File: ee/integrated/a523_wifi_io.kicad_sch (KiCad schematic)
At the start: 7 parts, among them U201 A523

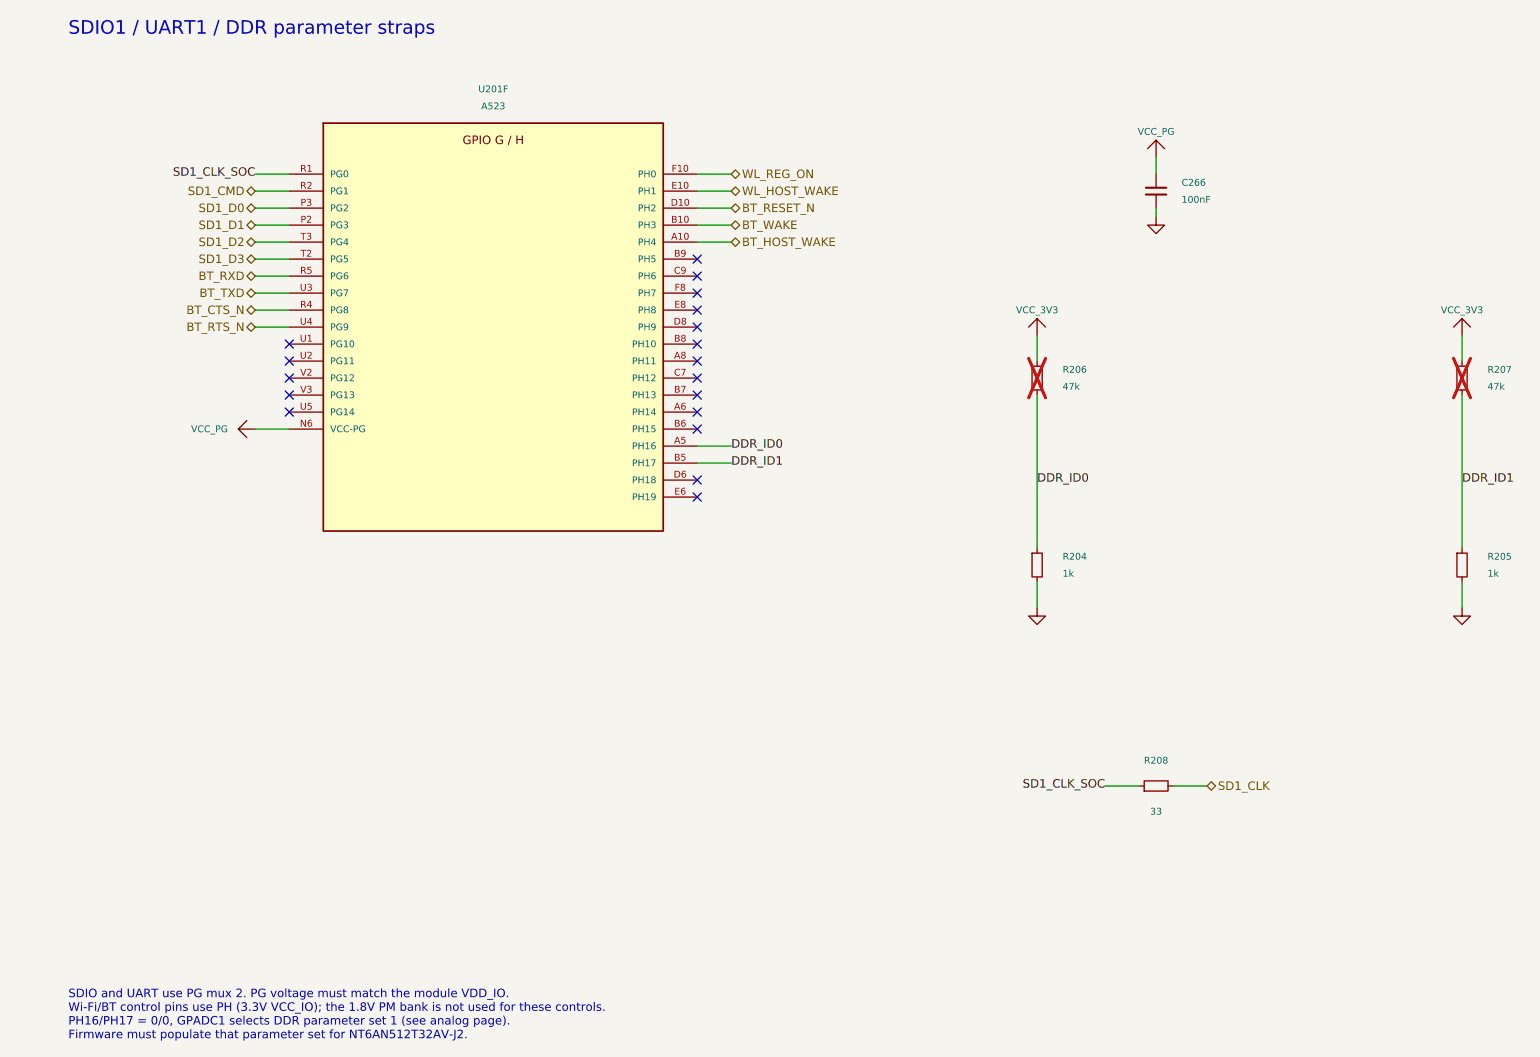
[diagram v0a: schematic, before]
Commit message: Working on the schematic.
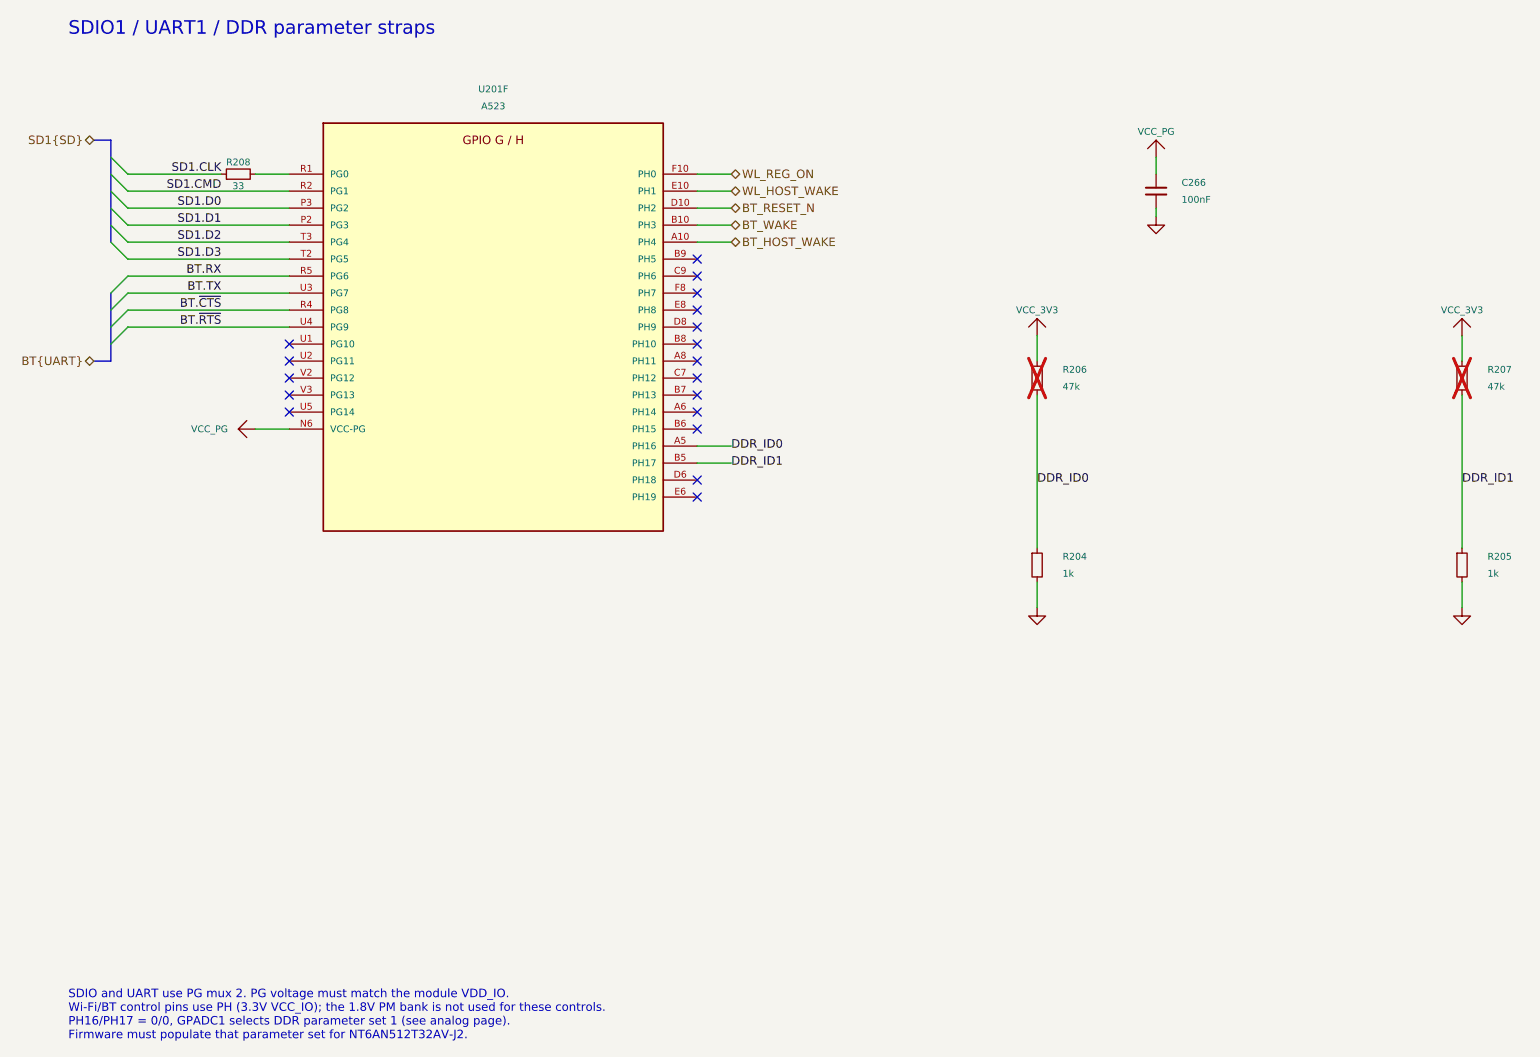
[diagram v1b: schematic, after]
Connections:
- net BT_CTS_N renamed BT.~{CTS}
- net BT_RTS_N renamed BT.~{RTS}
- net BT_RXD renamed BT.RX
- net BT_TXD renamed BT.TX
- net SD1_CLK: no longer names the net of R208.2
- net SD1_CLK: now also U201.R1 (PG0)
- net SD1_CLK_SOC renamed SD1.CLK
- net SD1.CLK: no longer U201.R1 (PG0)
- net SD1_CMD renamed SD1.CMD
- net SD1_D0 renamed SD1.D0
- net SD1_D1 renamed SD1.D1
- net SD1_D2 renamed SD1.D2
- net SD1_D3 renamed SD1.D3
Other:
- moved on the sheet: R208
